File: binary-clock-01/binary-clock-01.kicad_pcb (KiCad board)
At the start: 2 copper layers, 90 x 145 mm, 34 parts, among them SW100 SW_Push, SW101 SW_Push, U100 LF33_TO220, U101 ATTINY84-20PU, U102 cd4015b, U103 cd4015b

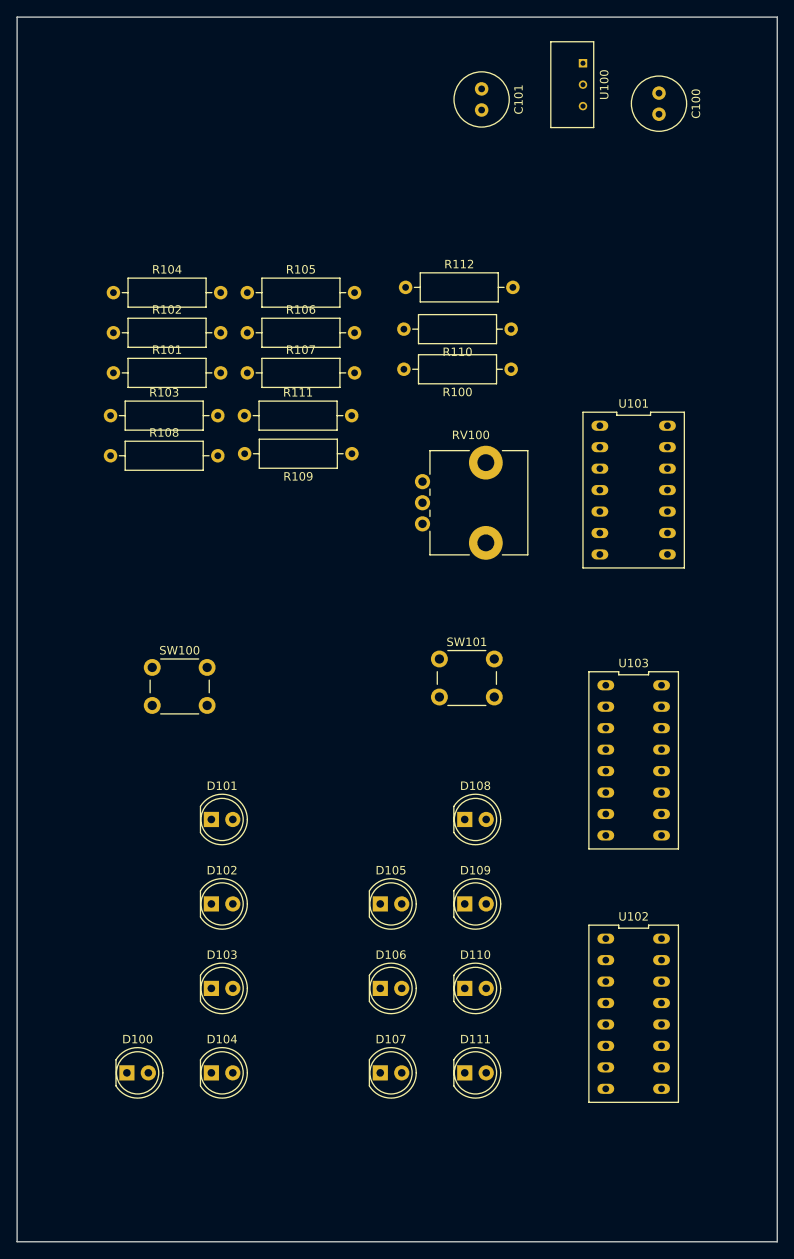
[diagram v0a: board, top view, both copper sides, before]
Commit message: finish pcb layout
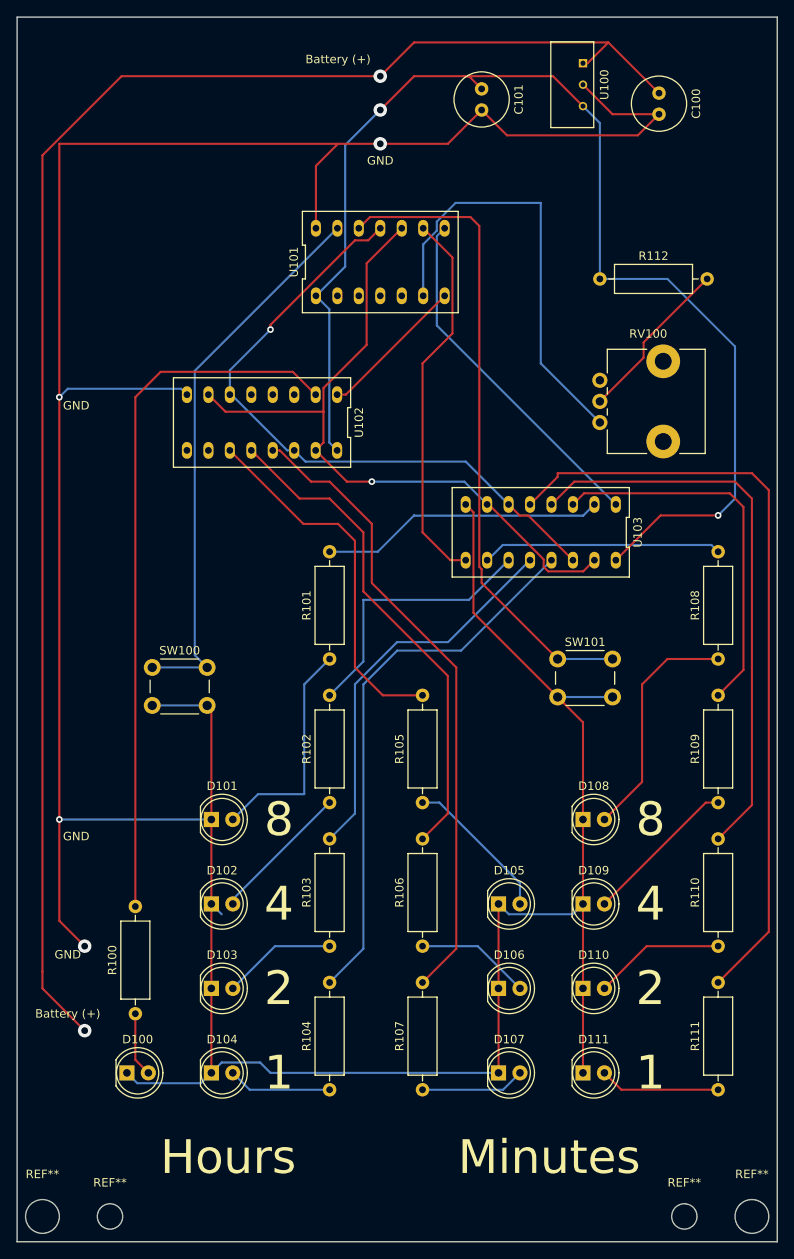
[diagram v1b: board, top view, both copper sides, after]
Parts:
- added REF**: MountingHole_4mm, MountingHole:MountingHole_4mm, F.Cu at (167.0, 172.0)
- added REF**: MountingHole_4mm, MountingHole:MountingHole_4mm, F.Cu at (83.0, 172.0)
- added REF**: MountingHole_3mm, MountingHole:MountingHole_3mm, F.Cu at (159.0, 172.0)
- added REF**: MountingHole_3mm, MountingHole:MountingHole_3mm, F.Cu at (91.0, 172.0)
- moved R104 97.8 mm to (117.0, 157.0), turned to 90 degrees
- moved R111 97.5 mm to (163.0, 157.0), turned to 90 degrees
- moved R100 88.3 mm to (94.0, 148.0), turned to 90 degrees
- moved R107 87.4 mm to (128.0, 157.0), turned to 90 degrees
- moved U102 82.7 mm to (109.0, 78.0), turned to 180 degrees
- moved R110 77.1 mm to (163.0, 140.0), turned to 90 degrees
- moved R108 75.9 mm to (163.0, 106.0), turned to 90 degrees
- moved R106 75.5 mm to (128.0, 140.0), turned to 90 degrees
- moved R103 68.0 mm to (117.0, 140.0), turned to 90 degrees
- moved R105 63.8 mm to (128.0, 123.0), turned to 90 degrees
- moved R102 61.2 mm to (117.0, 123.0), turned to 90 degrees
- moved R109 59.9 mm to (163.0, 123.0), turned to 90 degrees
- moved R101 42.5 mm to (117.0, 106.0), turned to 90 degrees
- moved U101 40.4 mm to (123.0, 59.0), turned to 0 degrees
- moved U103 29.2 mm to (142.0, 91.0), turned to 180 degrees
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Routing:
- net GND: track 0.00 -> 435.8 mm, vias 0 -> 4
- net +BATT: track 0.00 -> 190.7 mm, vias 0 -> 2
- net +3V3: track 0.00 -> 150.0 mm, vias 0 -> 2
- net /MM_D0_B0: track 0.00 -> 91.7 mm
- net /SR_DATA: track 0.00 -> 85.0 mm, vias 0 -> 1
- net /HH_D1_B0: track 0.00 -> 84.0 mm
- net Net-(SW101-Pad1): track 0.00 -> 76.9 mm
- net /SR_RESET: track 0.00 -> 76.7 mm, vias 0 -> 1
- net /MM_D1_B0: track 0.00 -> 75.4 mm
- net /MM_D0_B1: track 0.00 -> 67.6 mm
- net Net-(SW100-Pad1): track 0.00 -> 66.1 mm
- net /HH_D0_B0: track 0.00 -> 65.3 mm
- net /MM_D1_B1: track 0.00 -> 59.0 mm
- net Net-(RV100-Pad1): track 0.00 -> 51.6 mm
- net /HH_D0_B1: track 0.00 -> 46.4 mm
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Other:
- board text added: "1"
- board text added: "2"
- board text added: "4"
- board text added: "8"
- board text added: "Battery (+)"
- board text added: "GND"
- board text added: "Hours"
- board text added: "Minutes"
